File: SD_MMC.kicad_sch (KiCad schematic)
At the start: 6 parts, among them J2 Micro_SD_Card

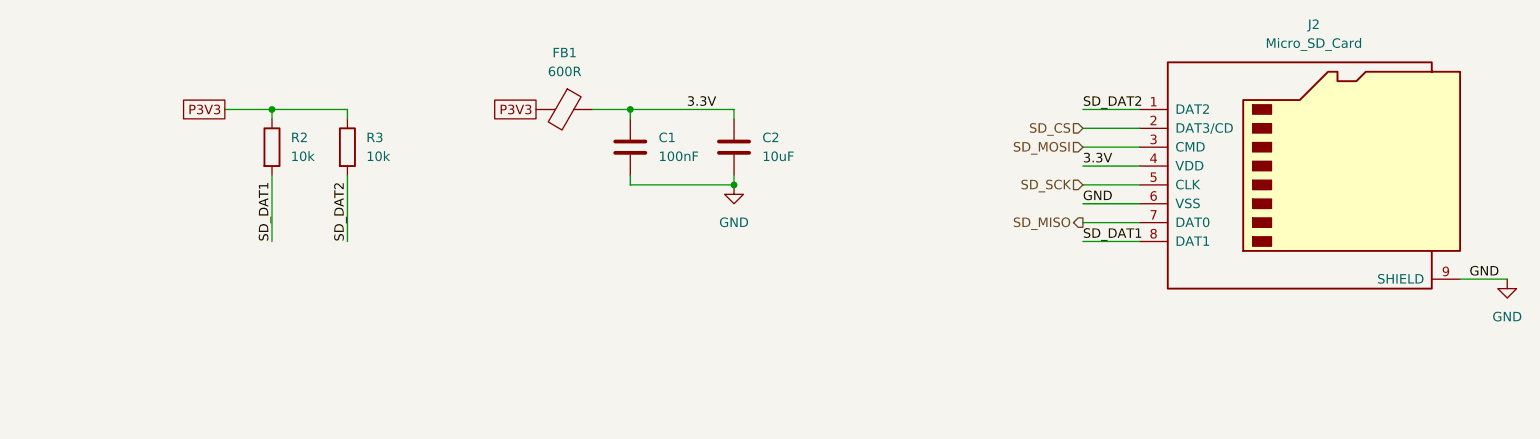
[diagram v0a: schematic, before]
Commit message: Power routed. Saving before reworking ICE40 pins to optimize layout
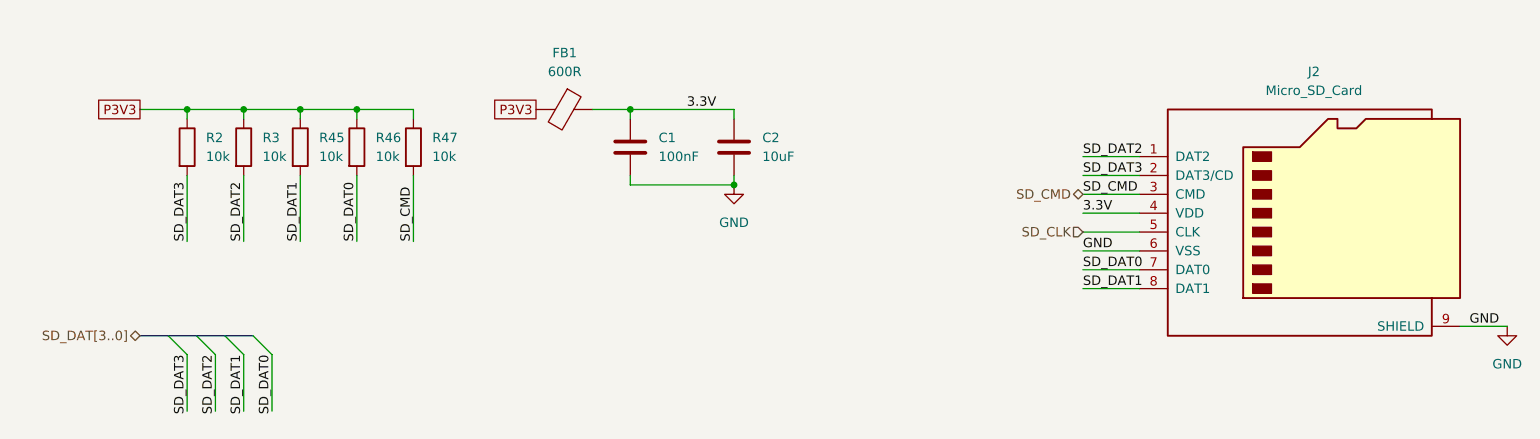
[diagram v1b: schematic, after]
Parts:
- added R45, R46, R47: 10k, Resistor_SMD:R_0603_1608Metric, symbol Device:R
- C1, C2: footprint (none) -> Capacitor_SMD:C_0603_1608Metric
- J2: footprint (none) -> Connector_Card:microSD_HC_Hirose_DM3BT-DSF-PEJS
- R2, R3: footprint (none) -> Resistor_SMD:R_0603_1608Metric
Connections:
- net P3V3: now also R45.1, R46.1, R47.1
- net SD_DAT1: now also R45.2; no longer R2.2
- net SD_CS renamed SD_DAT3
- net SD_DAT3: now also R2.2
- net SD_MISO renamed SD_DAT0
- net SD_DAT0: now also R46.2
- net SD_MOSI renamed SD_CMD
- net SD_CMD: now also R47.2
- net SD_SCK renamed SD_CLK
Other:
- moved on the sheet: J2, R2, R3

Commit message: Finished board. Added BOM
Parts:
- FB1: footprint (none) -> Capacitor_SMD:C_0603_1608Metric
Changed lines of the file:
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@@
 			)
 		)
-		(property "Footprint" ""
+		(property "Footprint" "Capacitor_SMD:C_0603_1608Metric"
 			(at 104.14 45.212 90)
 			(effects
